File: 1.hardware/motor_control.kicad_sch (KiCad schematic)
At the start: 0 parts

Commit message: 중간 저장
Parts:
- added C17: 4.7uF/10V, symbol Device:C_Small_US
- added J10: MOTOR_UVW, symbol Connector_Generic:Conn_01x03
- added J11: HALL_SENSOR, symbol Connector_Generic:Conn_01x05
- added R1, R97, R98: 0.2R, symbol Device:R_Shunt_US
- added U7, U8: LM2904D, PCM_Package_SO_AKL:SO-8_3.9x4.9mm_P1.27mm, symbol PCM_Amplifier_Operational_AKL:LM2904D
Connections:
- new net 5V: C17.1, J11.1 (Pin_1)
- new net GND: C17.2, J11.2 (Pin_2)
- new net HALL_A: J11.3 (Pin_3)
- new net HALL_B: J11.4 (Pin_4)
- new net HALL_C: J11.5 (Pin_5)
- new net MOTOR_U: J10.1 (Pin_1)
- new net MOTOR_V: J10.2 (Pin_2)
- new net MOTOR_W: J10.3 (Pin_3)

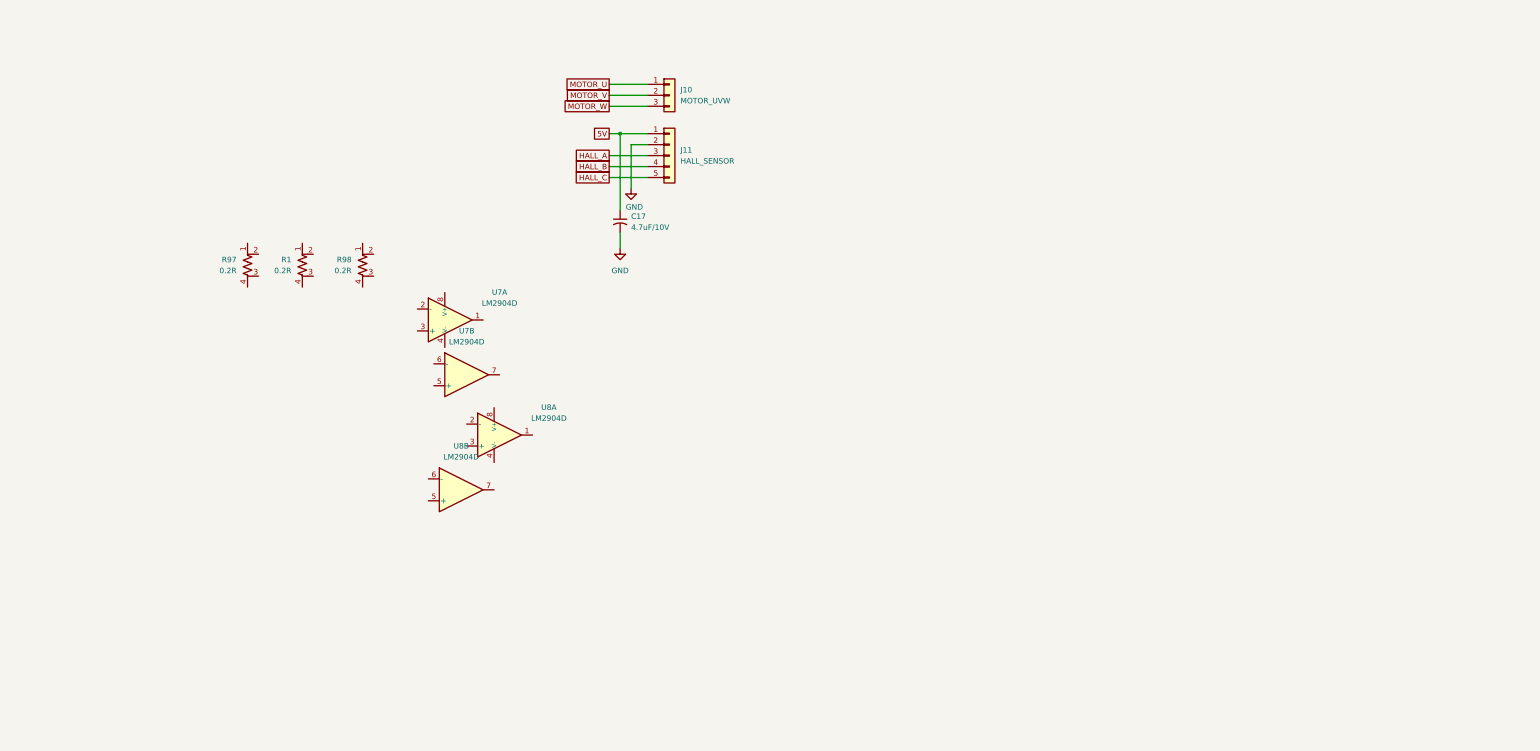
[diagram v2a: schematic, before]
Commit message: 중간 수정
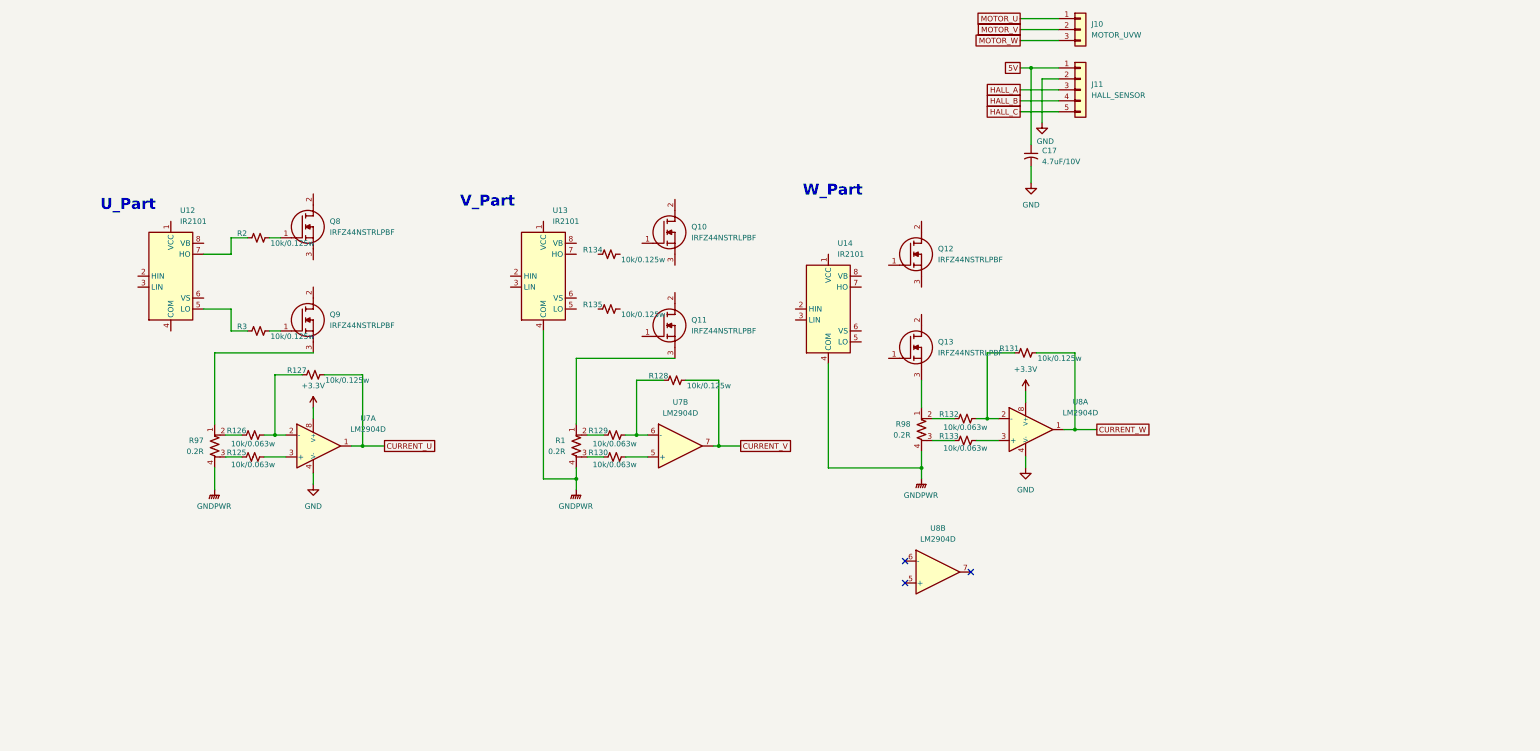
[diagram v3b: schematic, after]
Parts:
- added Q10, Q11, Q12, Q13, Q8, Q9: IRFZ44NSTRLPBF, SamacSys_Parts:IRFZ44NSTRLPBF, symbol SamacSys_Parts:IRFZ44NSTRLPBF
- added R125, R126, R129, R130, R132, R133: 10k/0.063w, symbol Device:R_Small_US
- added R127, R128, R131, R134, R135, R2, R3: 10k/0.125w, symbol Device:R_Small_US
- added U12, U13, U14: IR2101, symbol Driver_FET:IR2101
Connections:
- net GND: now also U7.4 (V-), U8.4 (V-)
- net at R98.1: now also Q13.3
- net at R98.2: now also R132.1
- net at R98.3: now also R133.1
- net GNDPWR: now reaches R98.4
- net GNDPWR: now also R1.4, R97.4, U13.4 (COM), U14.4 (COM)
- net CURRENT_W: now reaches U8.1
- net CURRENT_W: now also R131.2
- net at U8.2 (-): now also R131.1, R132.2
- net at U8.3 (+): now also R133.2
- net +3.3V: now reaches U8.8 (V+)
- net +3.3V: now also U7.8 (V+)
- net at R97.1: now also Q9.3
- net at R97.2: now also R126.1
- net at R97.3: now also R125.1
- net CURRENT_U: now reaches U7.1
- net CURRENT_U: now also R127.2
- net at U7.2 (-): now also R126.2, R127.1
- net at U7.3 (+): now also R125.2
- net at U7.5 (+): now also R130.2
- net at U7.6 (-): now also R128.1, R129.2
- net CURRENT_V: now reaches U7.7
- net CURRENT_V: now also R128.2
- net at R1.1: now also Q11.3
- net at R1.2: now also R129.1
- net at R1.3: now also R130.1
- new net: Q9.1, R3.2
- new net: R2.1, U12.7 (HO)
- new net: Q8.1, R2.2
- new net: R3.1, U12.5 (LO)
- no-connect marks 0 -> 3
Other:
- note added: "U_Part"
- note added: "V_Part"
- note added: "W_Part"
- moved on the sheet: C17, J10, J11, R1, R97, R98, U7A, U7B, U8A, U8B

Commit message: 중간 저장
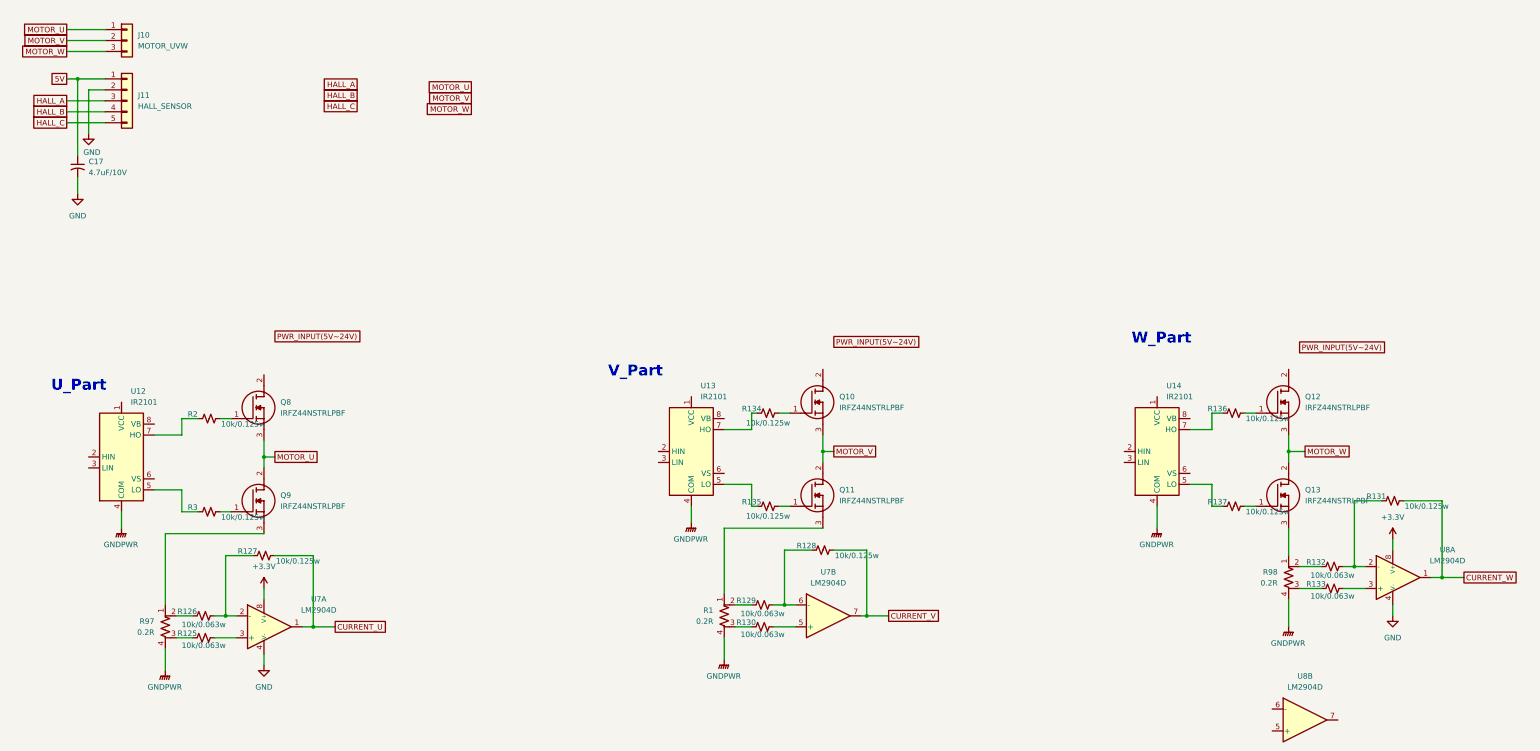
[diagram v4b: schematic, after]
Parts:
- added R136, R137: 10k/0.125w, symbol Device:R_Small_US
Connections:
- net GNDPWR: now also U12.4 (COM)
- net MOTOR_U: now also Q8.3, Q9.2
- net MOTOR_V: now also Q10.3, Q11.2
- net MOTOR_W: now also Q12.3, Q13.2
- net at Q10.1: now also R134.2
- net at U14.5 (LO): now also R137.1
- net at U14.7 (HO): now also R136.1
- net at R135.1: now also U13.5 (LO)
- net at R135.2: now also Q11.1
- net at U13.7 (HO): now also R134.1
- net at Q12.1: now also R136.2
- net at Q13.1: now also R137.2
- no-connect marks 3 -> 0
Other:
- moved on the sheet: C17, J10, J11, Q10, Q11, Q12, Q13, Q8, Q9, R1, R125, R126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

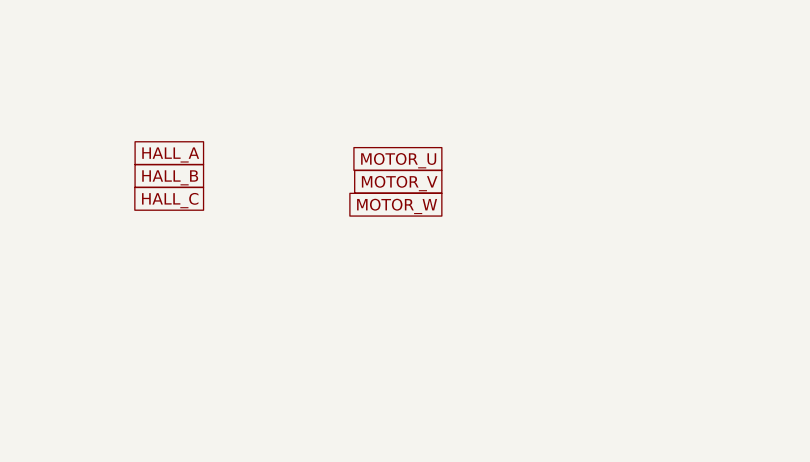
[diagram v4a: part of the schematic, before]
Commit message: 중간저장
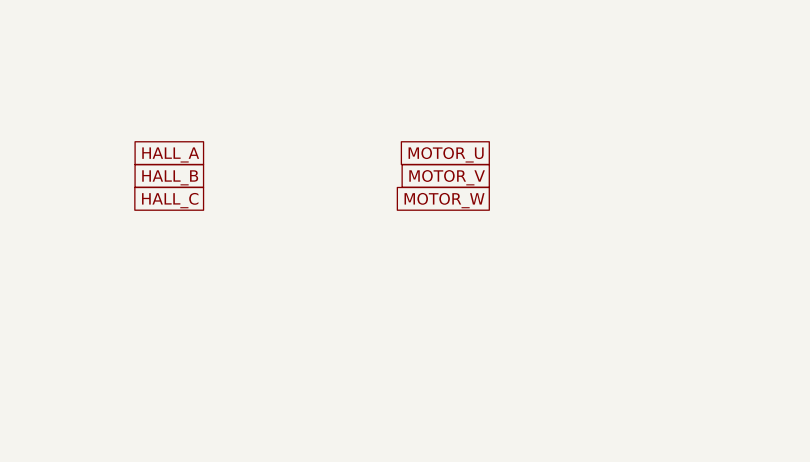
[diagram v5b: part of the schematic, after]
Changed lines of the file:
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@@
 	(global_label "MOTOR_U"
 		(shape passive)
-		(at 125.5383 38.7494 180)
+		(at 130.81 38.1 180)
 		(fields_autoplaced yes)
 		(effects
@@
 		)
 		(property "Intersheetrefs" "${INTERSHEET_REFS}"
-			(at 115.0163 38.7494 0)
+			(at 120.288 38.1 0)
 			(effects
 				(font
@@
 	(global_label "MOTOR_V"
 		(shape passive)
-		(at 125.5383 41.2894 180)
+		(at 130.81 40.64 180)
 		(fields_autoplaced yes)
 		(effects
@@
 		)
 		(property "Intersheetrefs" "${INTERSHEET_REFS}"
-			(at 115.2582 41.2894 0)
+			(at 120.5299 40.64 0)
 			(effects
 				(font
@@
 	(global_label "MOTOR_W"
 		(shape passive)
-		(at 125.5383 43.8294 180)
+		(at 130.81 43.18 180)
 		(fields_autoplaced yes)
 		(effects
@@
 		)
 		(property "Intersheetrefs" "${INTERSHEET_REFS}"
-			(at 114.8954 43.8294 0)
+			(at 120.1671 43.18 0)
 			(effects
 				(font
